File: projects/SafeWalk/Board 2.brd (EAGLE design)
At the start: 100 x 80 mm, 6 parts

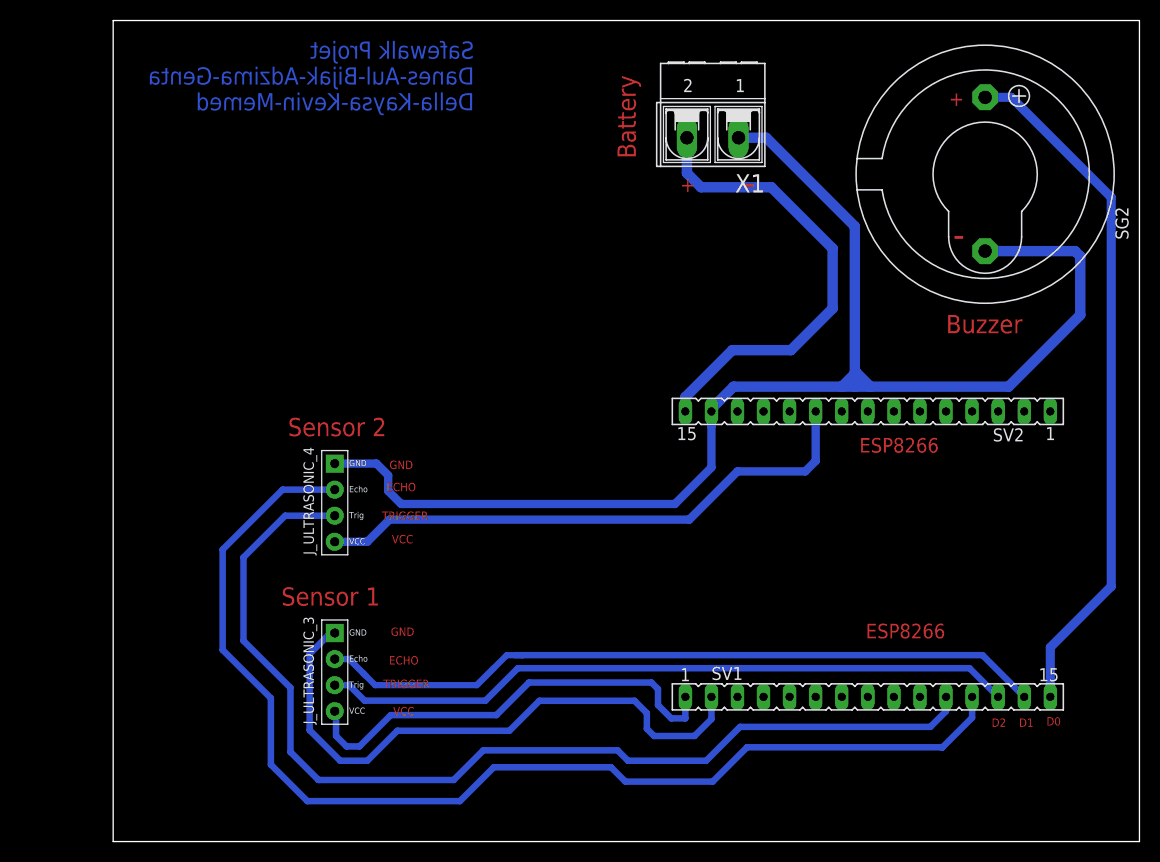
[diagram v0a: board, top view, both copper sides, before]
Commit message: upload malam ini
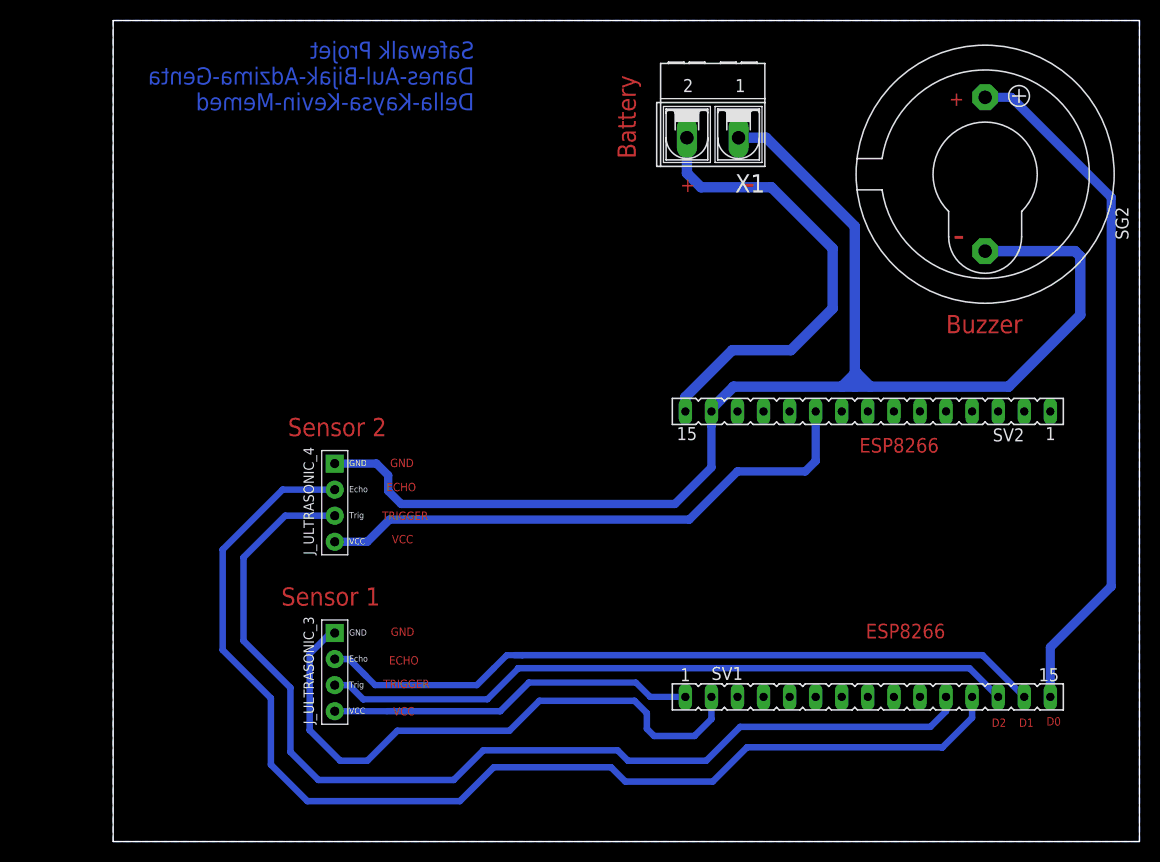
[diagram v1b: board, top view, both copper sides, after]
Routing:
- net N$4: track 44.0 -> 35.9 mm
- added copper zone on layer 16, net TEST
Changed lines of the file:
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@@
 <text x="76.581" y="38.608" size="1.4224" layer="1" align="center">ESP8266</text>
 <text x="28.194" y="20.447" size="0.8128" layer="1" align="center">GND</text>
-<text x="28.067" y="36.703" size="0.8128" layer="1" align="center">GND</text>
 <text x="28.321" y="17.653" size="0.8128" layer="1" align="center">ECHO</text>
 <text x="28.067" y="34.544" size="0.8128" layer="1" align="center">ECHO</text>
@@
 Danes-Aul-Bijak-Adzima-Genta
 Della-Kaysa-Kevin-Memed</text>
+<text x="28.134" y="36.896" size="0.8128" layer="1" align="center">GND</text>
 </plain>
 <attributes>
@@
 </class>
 </classes>
-<designrules name="default">
+<designrules name="default *">
 <description language="de">&lt;b&gt;EAGLE Design Rules&lt;/b&gt;
 &lt;p&gt;
@@
 <param name="mtCopper" value="0.035mm 0.035mm 0.035mm 0.035mm 0.035mm 0.035mm 0.035mm 0.035mm 0.035mm 0.035mm 0.035mm 0.035mm 0.035mm 0.035mm 0.035mm 0.035mm"/>
 <param name="mtIsolate" value="1.5mm 0.15mm 0.2mm 0.15mm 0.2mm 0.15mm 0.2mm 0.15mm 0.2mm 0.15mm 0.2mm 0.15mm 0.2mm 0.15mm 0.2mm"/>
-<param name="mdWireWire" value="6mil"/>
-<param name="mdWirePad" value="6mil"/>
-<param name="mdWireVia" value="6mil"/>
-<param name="mdPadPad" value="6mil"/>
-<param name="mdPadVia" value="6mil"/>
-<param name="mdViaVia" value="6mil"/>
-<param name="mdSmdPad" value="6mil"/>
-<param name="mdSmdVia" value="6mil"/>
-<param name="mdSmdSmd" value="6mil"/>
+<param name="mdWireWire" value="40mil"/>
+<param name="mdWirePad" value="40mil"/>
+<param name="mdWireVia" value="40mil"/>
+<param name="mdPadPad" value="40mil"/>
+<param name="mdPadVia" value="40mil"/>
+<param name="mdViaVia" value="40mil"/>
+<param name="mdSmdPad" value="40mil"/>
+<param name="mdSmdVia" value="40mil"/>
+<param name="mdSmdSmd" value="40mil"/>
 <param name="mdViaViaSameLayer" value="6mil"/>
 <param name="mnLayersViaInSmd" value="2"/>
@@
 <contactref element="J_ULTRASONIC_3" pad="TRIG"/>
 <wire x1="86.233" y1="14.097" x2="83.44" y2="16.89" width="0.635" layer="16"/>
-<wire x1="39.433" y1="16.89" x2="83.44" y2="16.89" width="0.635" layer="16"/>
+<wire x1="39.433" y1="16.89" x2="39.492" y2="16.89" width="0.635" layer="16"/>
+<wire x1="39.492" y1="16.89" x2="83.44" y2="16.89" width="0.635" layer="16"/>
 <wire x1="22.987" y1="15.24" x2="21.59" y2="15.24" width="0.635" layer="16"/>
-<wire x1="36.259" y1="13.716" x2="36.2715" y2="13.7285" width="0.635" layer="16"/>
-<wire x1="36.2715" y1="13.7285" x2="39.433" y2="16.89" width="0.635" layer="16"/>
-<wire x1="36.2715" y1="13.7285" x2="24.4985" y2="13.7285" width="0.635" layer="16"/>
-<wire x1="24.4985" y1="13.7285" x2="22.987" y2="15.24" width="0.635" layer="16"/>
+<wire x1="22.987" y1="15.24" x2="24.3675" y2="13.8595" width="0.635" layer="16"/>
+<wire x1="24.3715" y1="13.8555" x2="24.3675" y2="13.8595" width="0.635" layer="16"/>
+<wire x1="39.433" y1="16.827" x2="39.433" y2="16.89" width="0.6096" layer="16"/>
+<wire x1="39.492" y1="16.89" x2="36.4615" y2="13.8595" width="0.6096" layer="16"/>
+<wire x1="36.4615" y1="13.8595" x2="24.3675" y2="13.8595" width="0.6096" layer="16"/>
 </signal>
 <signal name="N$3">
@@
 <contactref element="SV1" pad="1"/>
 <contactref element="J_ULTRASONIC_3" pad="VCC"/>
-<wire x1="55.753" y1="12" x2="55.753" y2="14.097" width="0.635" layer="16"/>
-<wire x1="55.753" y1="12" x2="54.381" y2="12" width="0.635" layer="16"/>
-<wire x1="54.381" y1="12" x2="53.086" y2="13.295" width="0.635" layer="16"/>
-<wire x1="53.086" y1="13.295" x2="53.086" y2="14.859" width="0.635" layer="16"/>
-<wire x1="53.086" y1="14.859" x2="52.451" y2="15.494" width="0.635" layer="16"/>
-<wire x1="21.59" y1="12.7" x2="21.717" y2="12.573" width="0.635" layer="16"/>
-<wire x1="21.717" y1="12.573" x2="21.717" y2="10.287" width="0.635" layer="16"/>
-<wire x1="21.717" y1="10.287" x2="22.733" y2="9.271" width="0.635" layer="16"/>
-<wire x1="22.733" y1="9.271" x2="24.003" y2="9.271" width="0.635" layer="16"/>
-<wire x1="27.051" y1="12.319" x2="24.003" y2="9.271" width="0.635" layer="16"/>
-<wire x1="52.451" y1="15.494" x2="40.513" y2="15.494" width="0.635" layer="16"/>
-<wire x1="40.513" y1="15.494" x2="37.338" y2="12.319" width="0.635" layer="16"/>
-<wire x1="37.338" y1="12.319" x2="27.051" y2="12.319" width="0.635" layer="16"/>
+<wire x1="40.513" y1="15.494" x2="40.5095" y2="15.4905" width="0.635" layer="16"/>
+<wire x1="40.5095" y1="15.4905" x2="37.719" y2="12.7" width="0.635" layer="16"/>
+<wire x1="26.67" y1="12.7" x2="37.719" y2="12.7" width="0.635" layer="16"/>
+<wire x1="40.5095" y1="15.4905" x2="50.9305" y2="15.4905" width="0.6096" layer="16"/>
+<wire x1="50.9305" y1="15.4905" x2="52.324" y2="14.097" width="0.6096" layer="16"/>
+<wire x1="52.324" y1="14.097" x2="55.753" y2="14.097" width="0.6096" layer="16"/>
+<wire x1="26.67" y1="12.7" x2="21.59" y2="12.7" width="0.6096" layer="16"/>
 </signal>
 <signal name="N$5">
@@
 <wire x1="12.7" y1="27.686" x2="16.764" y2="31.75" width="0.635" layer="16"/>
 </signal>
+<signal name="TEST">
+<polygon width="1.016" layer="16">
+<vertex x="0" y="80"/>
+<vertex x="100" y="80"/>
+<vertex x="100" y="0"/>
+<vertex x="0" y="0"/>
+</polygon>
+<polygon width="1.27" layer="16">
+<vertex x="0" y="80"/>
+<vertex x="0" y="0"/>
+<vertex x="100" y="0"/>
+<vertex x="100" y="80"/>
+</polygon>
+</signal>
 </signals>
 <mfgpreviewcolors>
@@
 <mfgpreviewcolor name="substratecolor" color="0xFF786E46"/>
 </mfgpreviewcolors>
+<errors>
+</errors>
 </board>
 </drawing>
